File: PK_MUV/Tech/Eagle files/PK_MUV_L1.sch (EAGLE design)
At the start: 4 parts, among them U1 WS2812

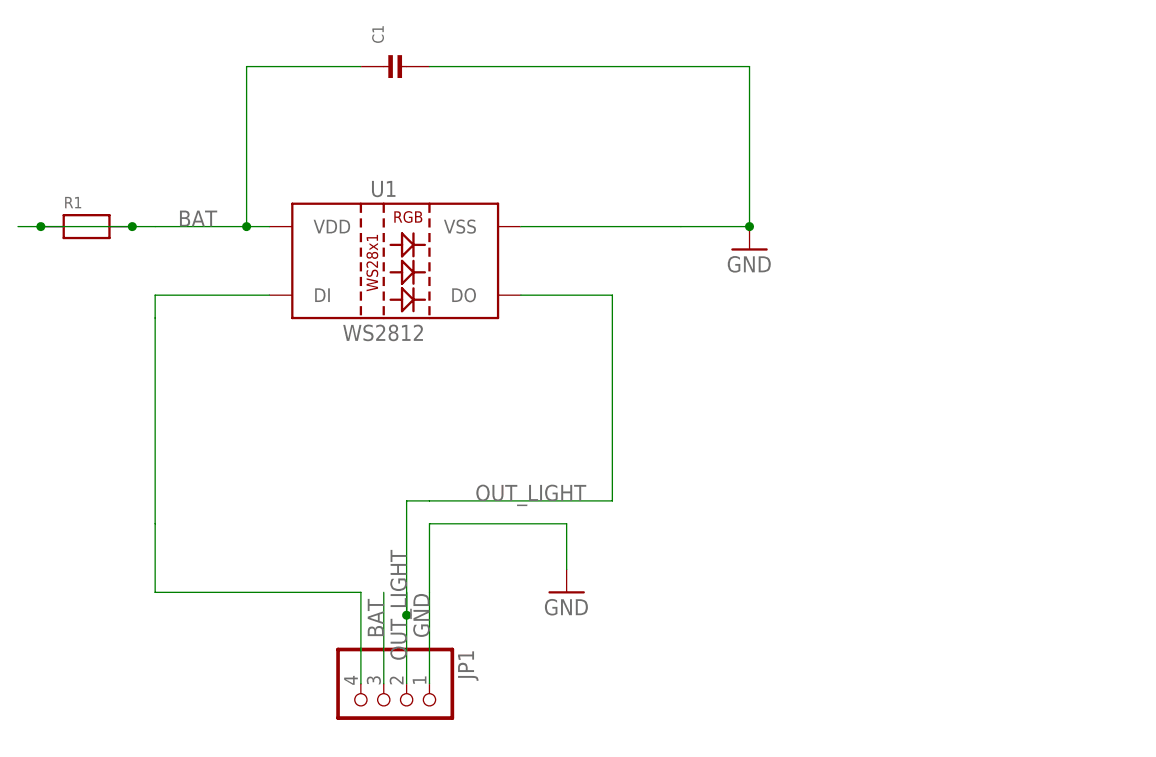
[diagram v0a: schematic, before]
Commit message: Update tech
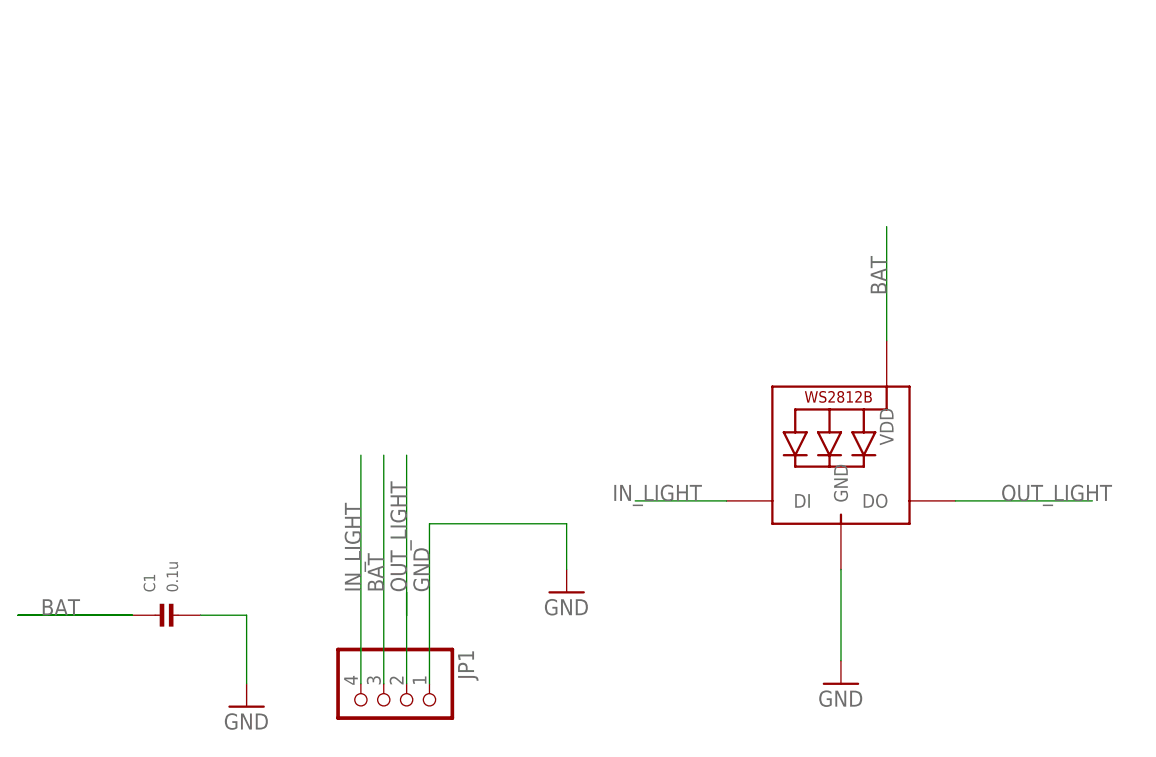
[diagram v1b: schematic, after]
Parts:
- removed R1: (no value), microbuilder:RESISTOR1206
- removed U1: WS2812, SparkFun-LED:WS2812"
- added LED1: WS2812B_5050N, adafruit:WS2812B_5050N
- C1: value (none) -> 0.1u
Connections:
- net BAT: now also LED1.VDD; no longer R1.1, R1.2, U1.VDD
- net GND: now also LED1.GND; no longer U1.VSS
- net IN_LIGHT: now also LED1.DI; no longer U1.DI
- net OUT_LIGHT: now also LED1.DO; no longer U1.DO
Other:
- moved on the sheet: C1
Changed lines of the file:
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@@
 <parts>
 <part name="GND1" library="supply1" library_urn="urn:adsk.eagle:library:371" deviceset="GND" device=""/>
-<part name="U1" library="SparkFun-LED" deviceset="WS2812" device="&quot;" value="WS2812"/>
 <part name="GND2" library="supply1" library_urn="urn:adsk.eagle:library:371" deviceset="GND" device=""/>
-<part name="C1" library="microbuilder" deviceset="CAP_CERAMIC" device="1206"/>
-<part name="R1" library="microbuilder" deviceset="RESISTOR" device="1206"/>
+<part name="C1" library="microbuilder" deviceset="CAP_CERAMIC" device="1206" value="0.1u"/>
 <part name="JP1" library="microbuilder" deviceset="HEADER-1X4" device=""/>
+<part name="LED1" library="adafruit" deviceset="WS2812B" device="_5050N"/>
+<part name="GND3" library="supply1" library_urn="urn:adsk.eagle:library:371" deviceset="GND" device=""/>
 </parts>
 <sheets>
@@
 <instances>
 <instance part="GND1" gate="1" x="58.42" y="48.26"/>
-<instance part="U1" gate="U1" x="40.64" y="83.82"/>
-<instance part="GND2" gate="1" x="78.74" y="86.36"/>
-<instance part="C1" gate="G$1" x="40.64" y="106.68" rot="R90"/>
-<instance part="R1" gate="G$1" x="5.08" y="88.9"/>
+<instance part="GND2" gate="1" x="22.86" y="35.56"/>
+<instance part="C1" gate="G$1" x="15.24" y="45.72" rot="R90"/>
 <instance part="JP1" gate="A" x="38.1" y="35.56" rot="R270"/>
+<instance part="LED1" gate="G$1" x="88.9" y="60.96"/>
+<instance part="GND3" gate="1" x="88.9" y="38.1"/>
 </instances>
 <busses>
@@
 <net name="BAT" class="1">
 <segment>
-<pinref part="U1" gate="U1" pin="VDD"/>
-<wire x1="25.4" y1="88.9" x2="22.86" y2="88.9" width="0.1524" layer="91"/>
-<label x="15.24" y="88.9" size="1.778" layer="95"/>
+<label x="0" y="45.72" size="1.778" layer="95"/>
 <pinref part="C1" gate="G$1" pin="P$1"/>
-<wire x1="22.86" y1="88.9" x2="12.7" y2="88.9" width="0.1524" layer="91"/>
-<wire x1="35.56" y1="106.68" x2="22.86" y2="106.68" width="0.1524" layer="91"/>
-<wire x1="22.86" y1="106.68" x2="22.86" y2="88.9" width="0.1524" layer="91"/>
-<junction x="22.86" y="88.9"/>
-<wire x1="12.7" y1="88.9" x2="10.16" y2="88.9" width="0.1524" layer="91"/>
-<wire x1="10.16" y1="88.9" x2="7.62" y2="88.9" width="0.1524" layer="91"/>
-<wire x1="-2.54" y1="88.9" x2="0" y2="88.9" width="0.1524" layer="91"/>
-<pinref part="R1" gate="G$1" pin="1"/>
-<wire x1="0" y1="88.9" x2="7.62" y2="88.9" width="0.1524" layer="91"/>
-<junction x="0" y="88.9"/>
-<pinref part="R1" gate="G$1" pin="2"/>
-<junction x="10.16" y="88.9"/>
+<wire x1="10.16" y1="45.72" x2="-2.54" y2="45.72" width="0.1524" layer="91"/>
+<wire x1="-2.54" y1="45.72" x2="10.16" y2="45.72" width="0.1524" layer="91"/>
+<wire x1="-2.54" y1="45.72" x2="10.16" y2="45.72" width="0.1524" layer="91"/>
 </segment>
 <segment>
 <pinref part="JP1" gate="A" pin="3"/>
-<wire x1="38.1" y1="38.1" x2="38.1" y2="48.26" width="0.1524" layer="91"/>
-<label x="38.1" y="43.18" size="1.778" layer="95" rot="R90"/>
+<wire x1="38.1" y1="38.1" x2="38.1" y2="63.5" width="0.1524" layer="91"/>
+<label x="38.1" y="48.26" size="1.778" layer="95" rot="R90"/>
+</segment>
+<segment>
+<pinref part="LED1" gate="G$1" pin="VDD"/>
+<wire x1="93.98" y1="76.2" x2="93.98" y2="88.9" width="0.1524" layer="91"/>
+<label x="93.98" y="81.28" size="1.778" layer="95" rot="R90"/>
 </segment>
 </net>
 <net name="IN_LIGHT" class="0">
 <segment>
-<wire x1="12.7" y1="55.88" x2="12.7" y2="78.74" width="0.1524" layer="91"/>
-<pinref part="U1" gate="U1" pin="DI"/>
-<wire x1="12.7" y1="78.74" x2="12.7" y2="81.28" width="0.1524" layer="91"/>
-<wire x1="12.7" y1="81.28" x2="25.4" y2="81.28" width="0.1524" layer="91"/>
-<wire x1="12.7" y1="55.88" x2="12.7" y2="48.26" width="0.1524" layer="91"/>
-<wire x1="12.7" y1="48.26" x2="35.56" y2="48.26" width="0.1524" layer="91"/>
 <pinref part="JP1" gate="A" pin="4"/>
-<wire x1="35.56" y1="48.26" x2="35.56" y2="38.1" width="0.1524" layer="91"/>
+<wire x1="35.56" y1="63.5" x2="35.56" y2="38.1" width="0.1524" layer="91"/>
+<label x="35.56" y="48.26" size="1.778" layer="95" rot="R90"/>
+</segment>
+<segment>
+<pinref part="LED1" gate="G$1" pin="DI"/>
+<wire x1="76.2" y1="58.42" x2="66.04" y2="58.42" width="0.1524" layer="91"/>
+<label x="63.5" y="58.42" size="1.778" layer="95"/>
 </segment>
 </net>
@@
 <pinref part="JP1" gate="A" pin="1"/>
 <wire x1="43.18" y1="38.1" x2="43.18" y2="48.26" width="0.1524" layer="91"/>
-<label x="43.18" y="43.18" size="1.778" layer="95" rot="R90"/>
+<label x="43.18" y="48.26" size="1.778" layer="95" rot="R90"/>
 <wire x1="43.18" y1="48.26" x2="43.18" y2="55.88" width="0.1524" layer="91"/>
 </segment>
 <segment>
-<pinref part="U1" gate="U1" pin="VSS"/>
-<wire x1="53.34" y1="88.9" x2="71.12" y2="88.9" width="0.1524" layer="91"/>
 <pinref part="GND2" gate="1" pin="GND"/>
-<wire x1="71.12" y1="88.9" x2="78.74" y2="88.9" width="0.1524" layer="91"/>
 <pinref part="C1" gate="G$1" pin="P$2"/>
-<wire x1="43.18" y1="106.68" x2="78.74" y2="106.68" width="0.1524" layer="91"/>
-<wire x1="78.74" y1="106.68" x2="78.74" y2="88.9" width="0.1524" layer="91"/>
-<junction x="78.74" y="88.9"/>
+<wire x1="17.78" y1="45.72" x2="22.86" y2="45.72" width="0.1524" layer="91"/>
+<wire x1="22.86" y1="45.72" x2="22.86" y2="38.1" width="0.1524" layer="91"/>
+</segment>
+<segment>
+<pinref part="LED1" gate="G$1" pin="GND"/>
+<wire x1="88.9" y1="50.8" x2="88.9" y2="40.64" width="0.1524" layer="91"/>
+<pinref part="GND3" gate="1" pin="GND"/>
 </segment>
 </net>
 <net name="OUT_LIGHT" class="0">
 <segment>
-<wire x1="43.18" y1="58.42" x2="63.5" y2="58.42" width="0.1524" layer="91"/>
-<label x="48.26" y="58.42" size="1.778" layer="95"/>
-<pinref part="U1" gate="U1" pin="DO"/>
-<wire x1="53.34" y1="81.28" x2="63.5" y2="81.28" width="0.1524" layer="91"/>
-<wire x1="63.5" y1="81.28" x2="63.5" y2="58.42" width="0.1524" layer="91"/>
 <pinref part="JP1" gate="A" pin="2"/>
 <wire x1="40.64" y1="38.1" x2="40.64" y2="45.72" width="0.1524" layer="91"/>
-<label x="40.64" y="40.64" size="1.778" layer="95" rot="R90"/>
+<label x="40.64" y="48.26" size="1.778" layer="95" rot="R90"/>
 <wire x1="40.64" y1="45.72" x2="40.64" y2="48.26" width="0.1524" layer="91"/>
-<wire x1="43.18" y1="58.42" x2="40.64" y2="58.42" width="0.1524" layer="91"/>
-<wire x1="40.64" y1="58.42" x2="40.64" y2="45.72" width="0.1524" layer="91"/>
-<junction x="40.64" y="45.72"/>
+<wire x1="40.64" y1="63.5" x2="40.64" y2="45.72" width="0.1524" layer="91"/>
+</segment>
+<segment>
+<pinref part="LED1" gate="G$1" pin="DO"/>
+<wire x1="101.6" y1="58.42" x2="116.84" y2="58.42" width="0.1524" layer="91"/>
+<label x="106.68" y="58.42" size="1.778" layer="95"/>
 </segment>
 </net>
